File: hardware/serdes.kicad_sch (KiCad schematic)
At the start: 22 parts, among them Q3 BSS138, U4 CCGM1A1, X2 100 MHz LVDS 3.2x2.5

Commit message: Routing
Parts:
- Q3: footprint Package_TO_SOT_SMD:SOT-23 -> Package_TO_SOT_SMD:SOT-523
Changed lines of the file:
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@@
 			)
 		)
-		(property "Footprint" "Package_TO_SOT_SMD:SOT-23"
+		(property "Footprint" "Package_TO_SOT_SMD:SOT-523"
 			(at 191.135 113.03 0)
 			(effects

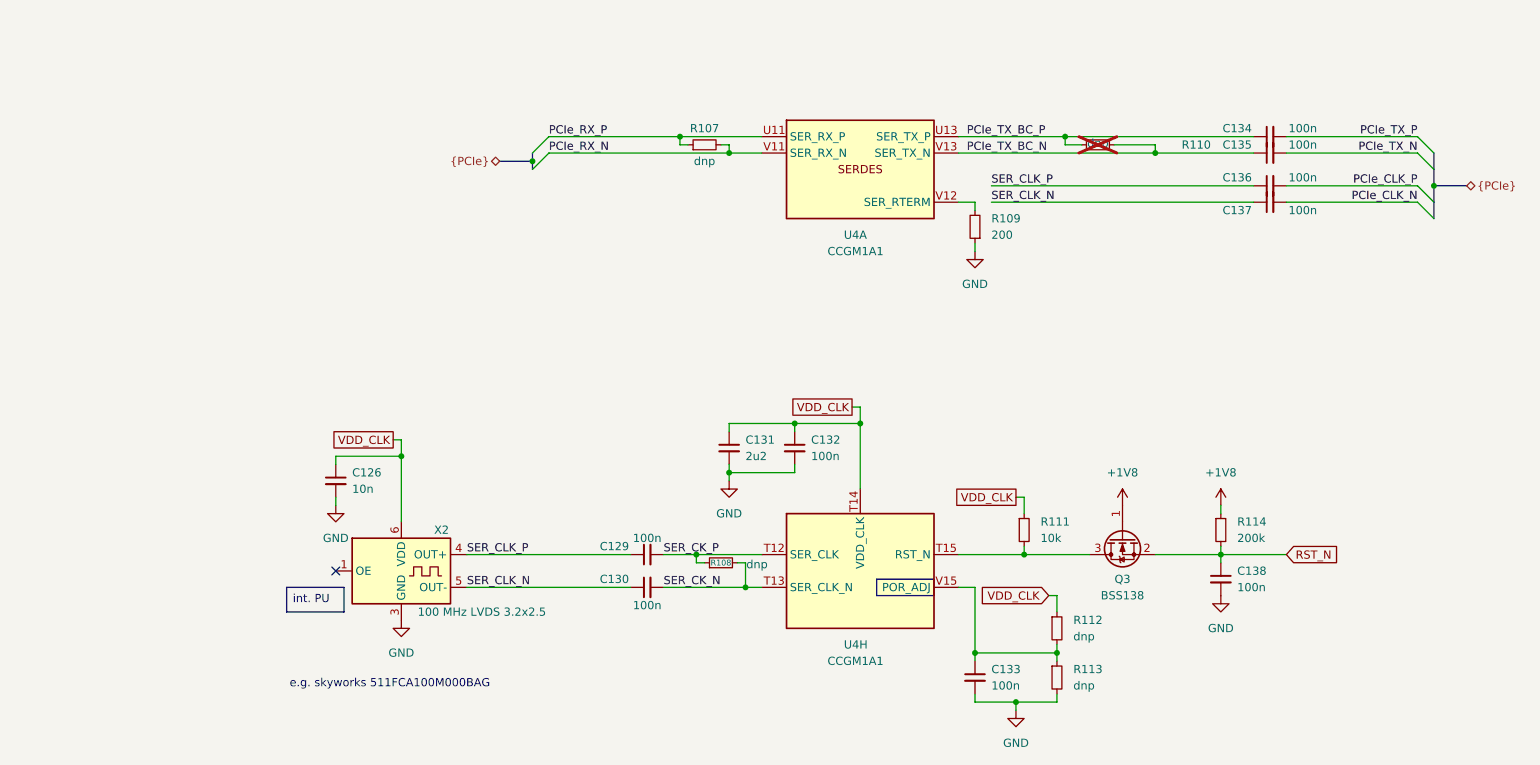
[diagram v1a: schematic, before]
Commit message: Cleanup
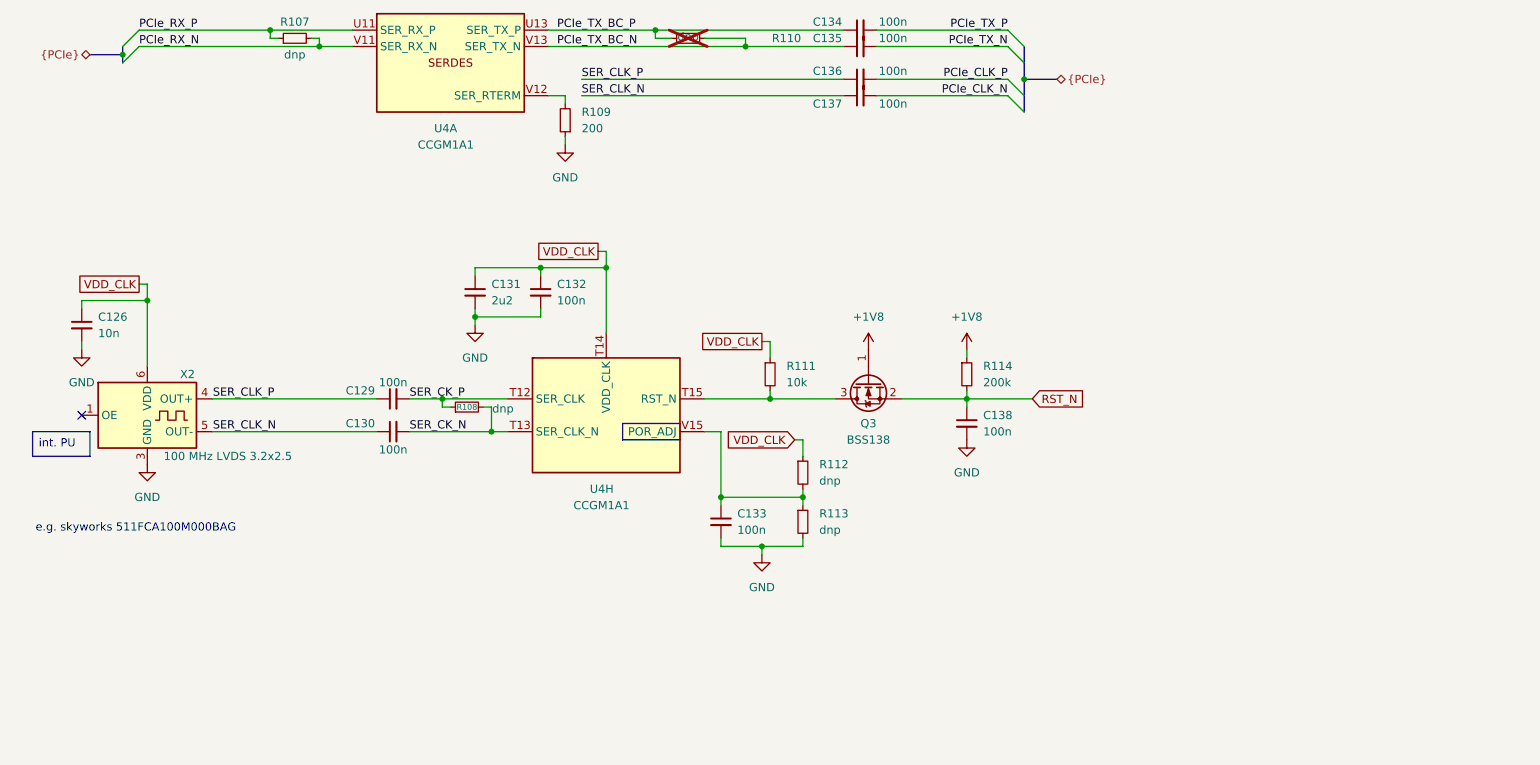
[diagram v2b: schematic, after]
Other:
- moved on the sheet: C126, C129, C130, C131, C132, C133, C134, C135, C136, C137, C138, Q3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
